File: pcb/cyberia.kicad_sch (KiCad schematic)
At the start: 109 parts, among them J1 USB_C_Receptacle_USB2.0_16P, SW10 SW_Push, SW11 SW_Push, SW12 SW_Push, SW13 SW_Push, SW14 SW_Push, SW15 SW_Push, SW16 SW_Push, SW17 SW_Push, SW18 SW_Push, SW19 SW_Push, SW2 SW_Push, SW21 SW_Push, SW22 SW_Push, SW23 SW_Push, SW24 SW_Push, SW25 SW_Push, SW26 SW_Push, SW27 SW_Push, SW28 SW_Push, SW29 SW_Push, SW3 SW_Push, SW30 SW_Push, SW31 SW_Push, SW32 SW_Push, SW33 SW_Push, SW34 SW_Push, SW35 SW_Push, SW36 SW_Push, SW37 SW_Push, SW38 SW_Push, SW39 Reset, SW4 SW_Push, SW40 ROM, SW5 SW_Push, SW6 SW_Push, SW7 SW_Push, SW8 SW_Push, SW9 SW_Push, U1 RP2040, U2 AP2127N-3.3, U3 USBLC6-2SC6, U4 MX25R3235FZNxx0, Y1 Crystal_GND24

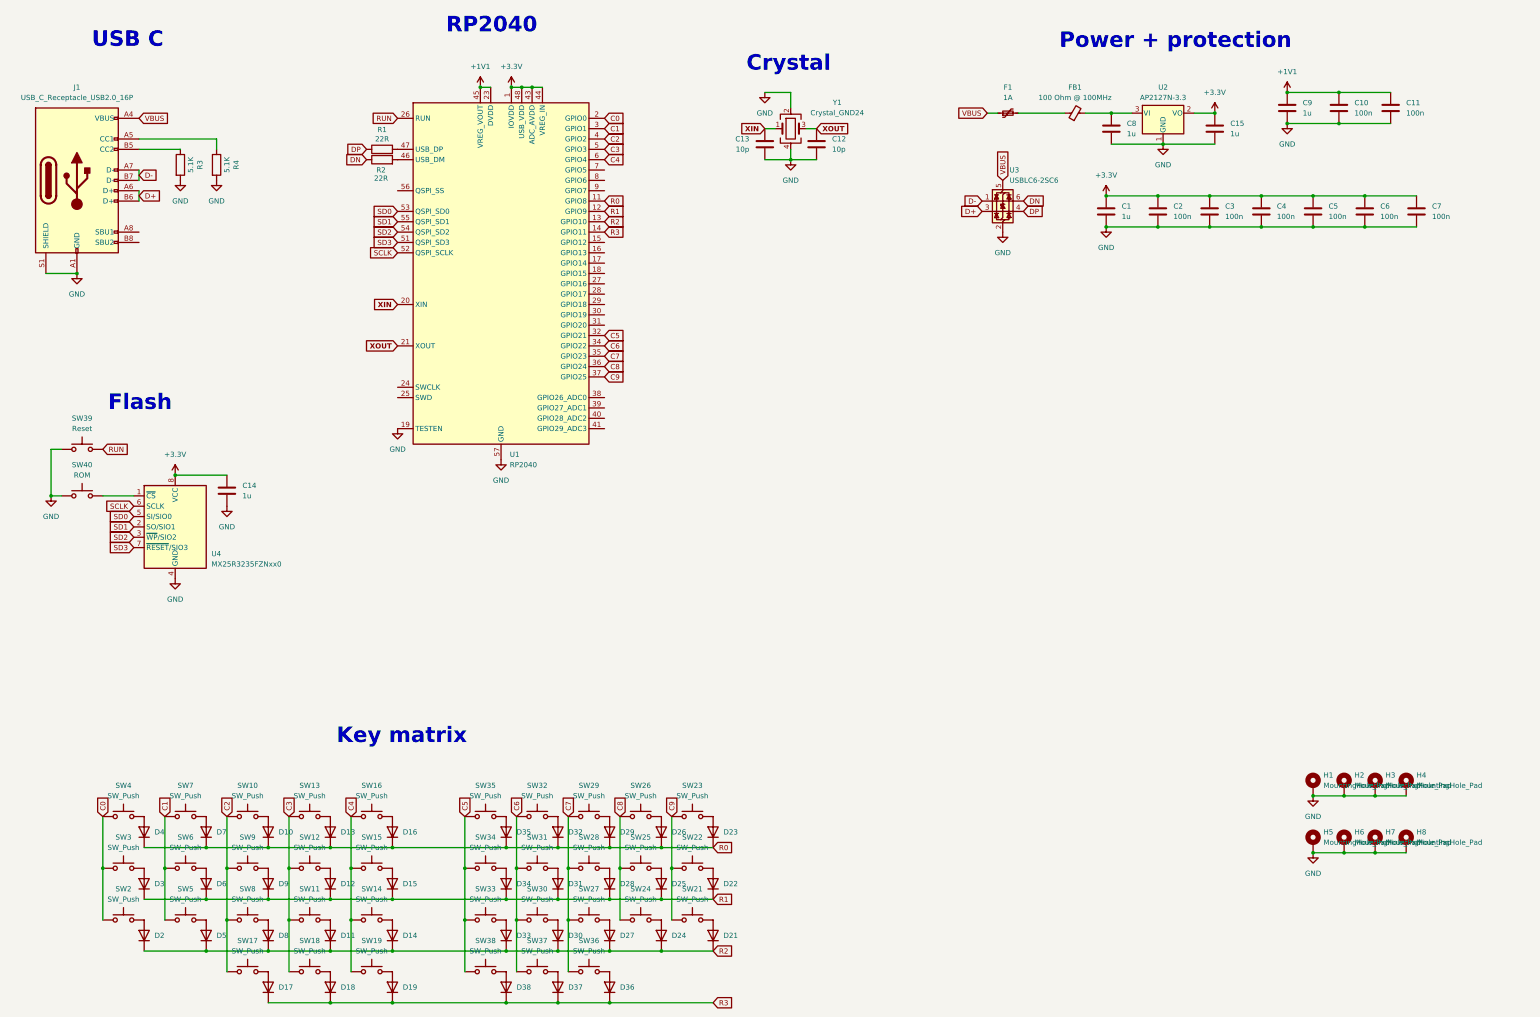
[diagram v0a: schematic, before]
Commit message: rev.666
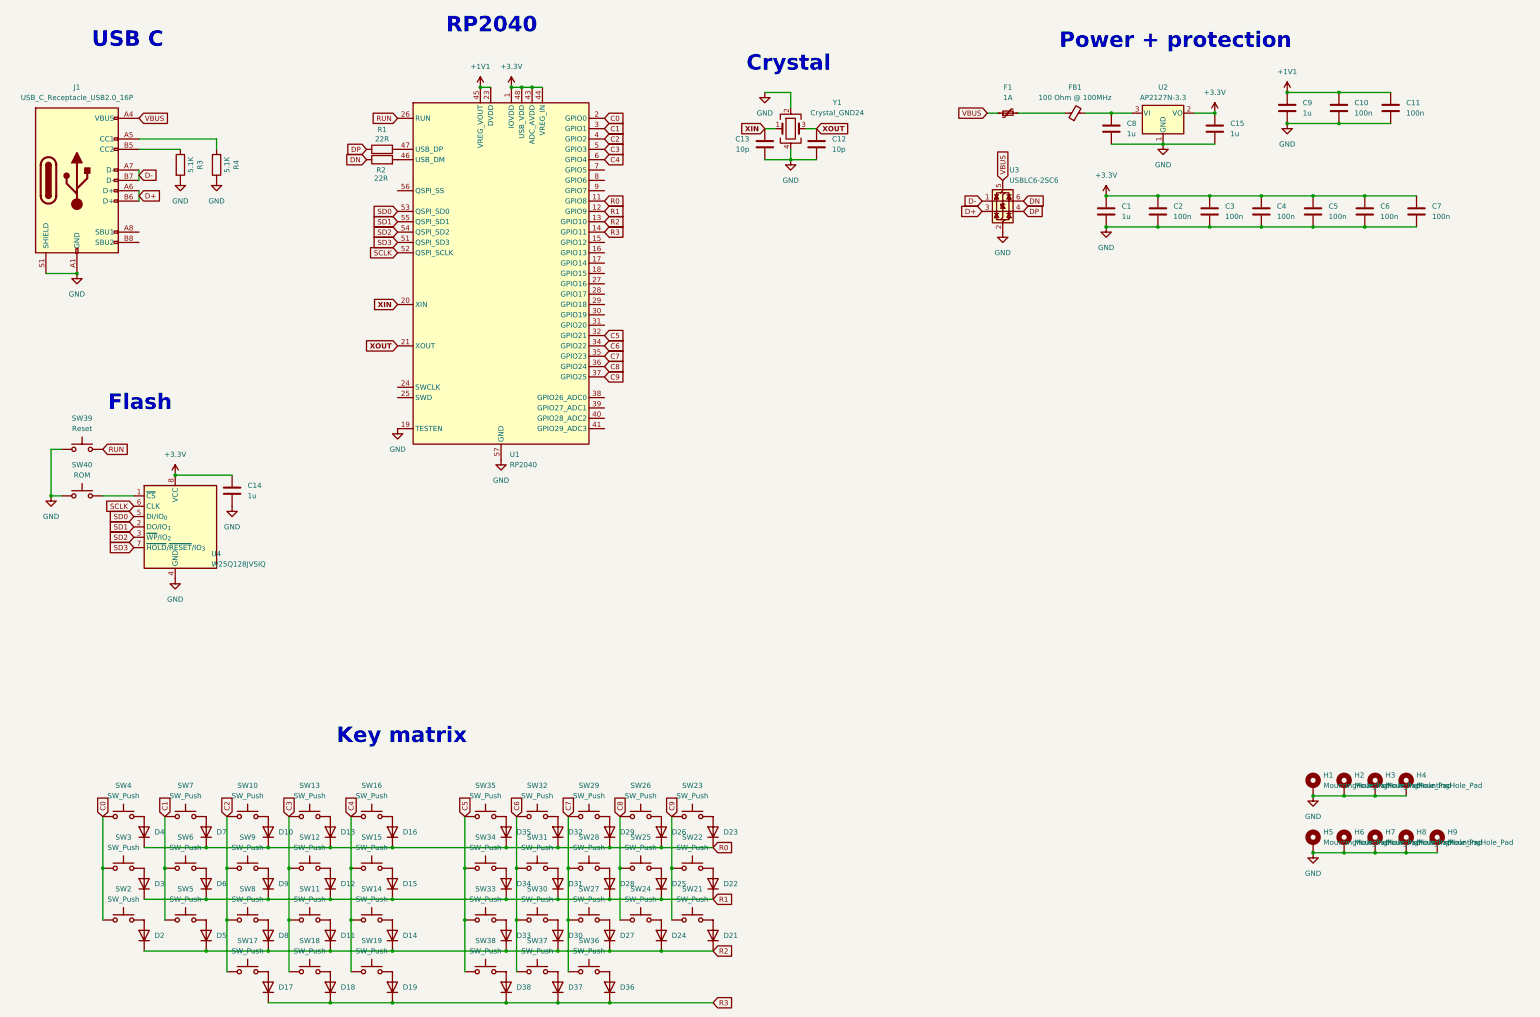
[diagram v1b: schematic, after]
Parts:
- added H9: MountingHole_Pad, MountingHole:MountingHole_3.2mm_M3, symbol Mechanical:MountingHole_Pad
- C1, C14, C15, C8, C9: LCSC (none) -> C1592
- C10, C11, C2, C3, C4, C5, C6, C7: LCSC (none) -> C1590
- C12, C13: LCSC (none) -> C1634
- D10, D11, D12, D13, D14, D15, D16, D17, D18, D19, D2, D21, D22, D23, D24, D25, D26, D27, D28, D29, D3, D30, D31, D32, D33, D34, D35, D36, D37, D38, D4, D5, D6, D7, D8, D9: LCSC (none) -> C68883
- F1: footprint Fuse:Fuse_0603_1608Metric -> Fuse:Fuse_0805_2012Metric; LCSC (none) -> C20980
- FB1: footprint Resistor_SMD:R_0603_1608Metric -> Resistor_SMD:R_0805_2012Metric; LCSC (none) -> C1015
- J1: LCSC (none) -> C2894897
- R1, R2: LCSC (none) -> C23345
- R3, R4: LCSC (none) -> C23186
- U1: LCSC (none) -> C2040
- U2: LCSC (none) -> C176954
- U3: LCSC (none) -> C7519
- U4: value MX25R3235FZNxx0 -> W25Q128JVSIQ; footprint Package_SON:WSON-8-1EP_6x5mm_P1.27mm_EP3.4x4mm -> Package_SO:SOIC-8_5.3x5.3mm_P1.27mm; symbol Memory_Flash:MX25R3235FZNxx0 -> Memory_Flash:W25Q128JVS; LCSC (none) -> C97521
- Y1: LCSC (none) -> C20625731
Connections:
- net GND: now also H9.1; no longer U4.9 (GND)
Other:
- moved on the sheet: C14, U4
